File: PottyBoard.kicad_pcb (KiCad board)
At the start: 2 copper layers, 20.3 x 10.2 mm, 12 parts, among them J1 Conn_01x03, J2 Conn_01x03, U1 LMV358

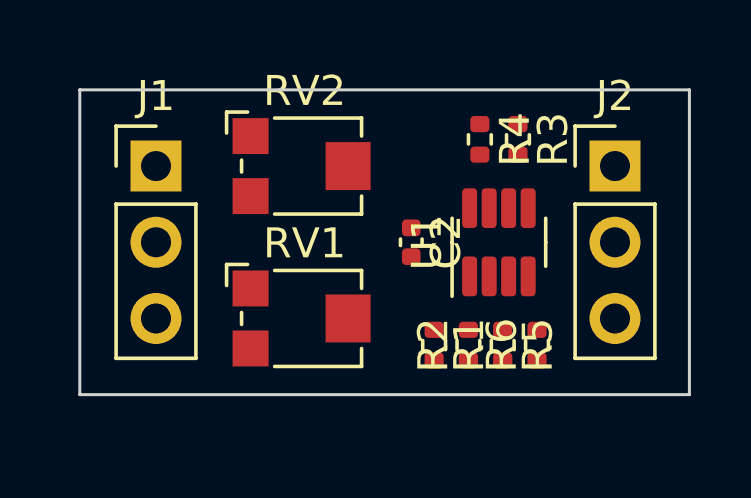
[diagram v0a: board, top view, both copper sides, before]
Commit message: PCB layout
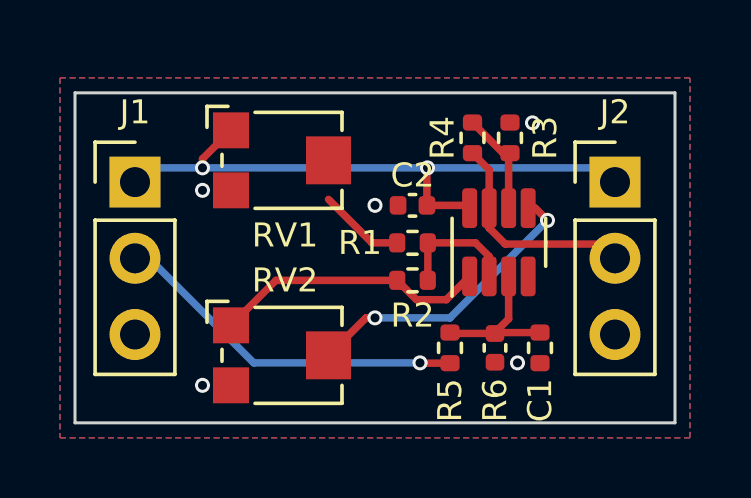
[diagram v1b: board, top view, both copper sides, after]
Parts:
- added C1: 10n, Capacitor_SMD:C_0402_1005Metric, F.Cu at (151.0, 97.5)
- moved RV2 6.34 mm to (144.0, 97.8)
- moved RV1 5.31 mm to (144.0, 91.2)
- moved R1 3.48 mm to (148.2, 94.0), turned to 0 degrees
- moved R2 2.85 mm to (148.2, 95.2), turned to 180 degrees
- moved R5 1.76 mm to (149.5, 97.5)
- moved C2 1.23 mm to (148.2, 92.8), turned to 180 degrees
- moved J1 0.88 mm to (139.0, 92.0)
- moved J2 0.53 mm to (155.0, 92.0)
- moved R3 0.27 mm to (151.5, 90.5)
- moved R4 0.25 mm to (150.2, 90.5)
- moved R6 0.14 mm to (152.5, 97.5)
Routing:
- net VCC: track 0.00 -> 20.4 mm, vias 0 -> 2
- net Net-(J1-Pin_2): track 0.00 -> 12.1 mm, vias 0 -> 1
- net Net-(U1B-+): track 0.00 -> 9.98 mm, vias 0 -> 2
- net Net-(R2-Pad2): track 0.00 -> 9.17 mm
- net Net-(J2-Pin_2): track 0.00 -> 7.14 mm
- net Net-(U1A-+): track 0.00 -> 5.07 mm
- net Net-(U1A--): track 0.00 -> 4.15 mm
- net Net-(U1B--): track 0.00 -> 3.52 mm
- net Net-(R1-Pad1): track 0.00 -> 2.89 mm
- net GND: vias 0 -> 5
- added copper zone on B.Cu, net GND
- added copper zone on F.Cu, net GND
- added copper zone on In1.Cu, net GND
- added copper zone on In2.Cu, net GND
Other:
- board size 20.3 x 10.2 mm -> 20 x 11 mm
- copper layers 2 -> 4
